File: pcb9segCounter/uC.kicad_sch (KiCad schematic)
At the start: 14 parts, among them J1 AVR-ISP-6, J2 SAO, U1 ATtiny84A-SS

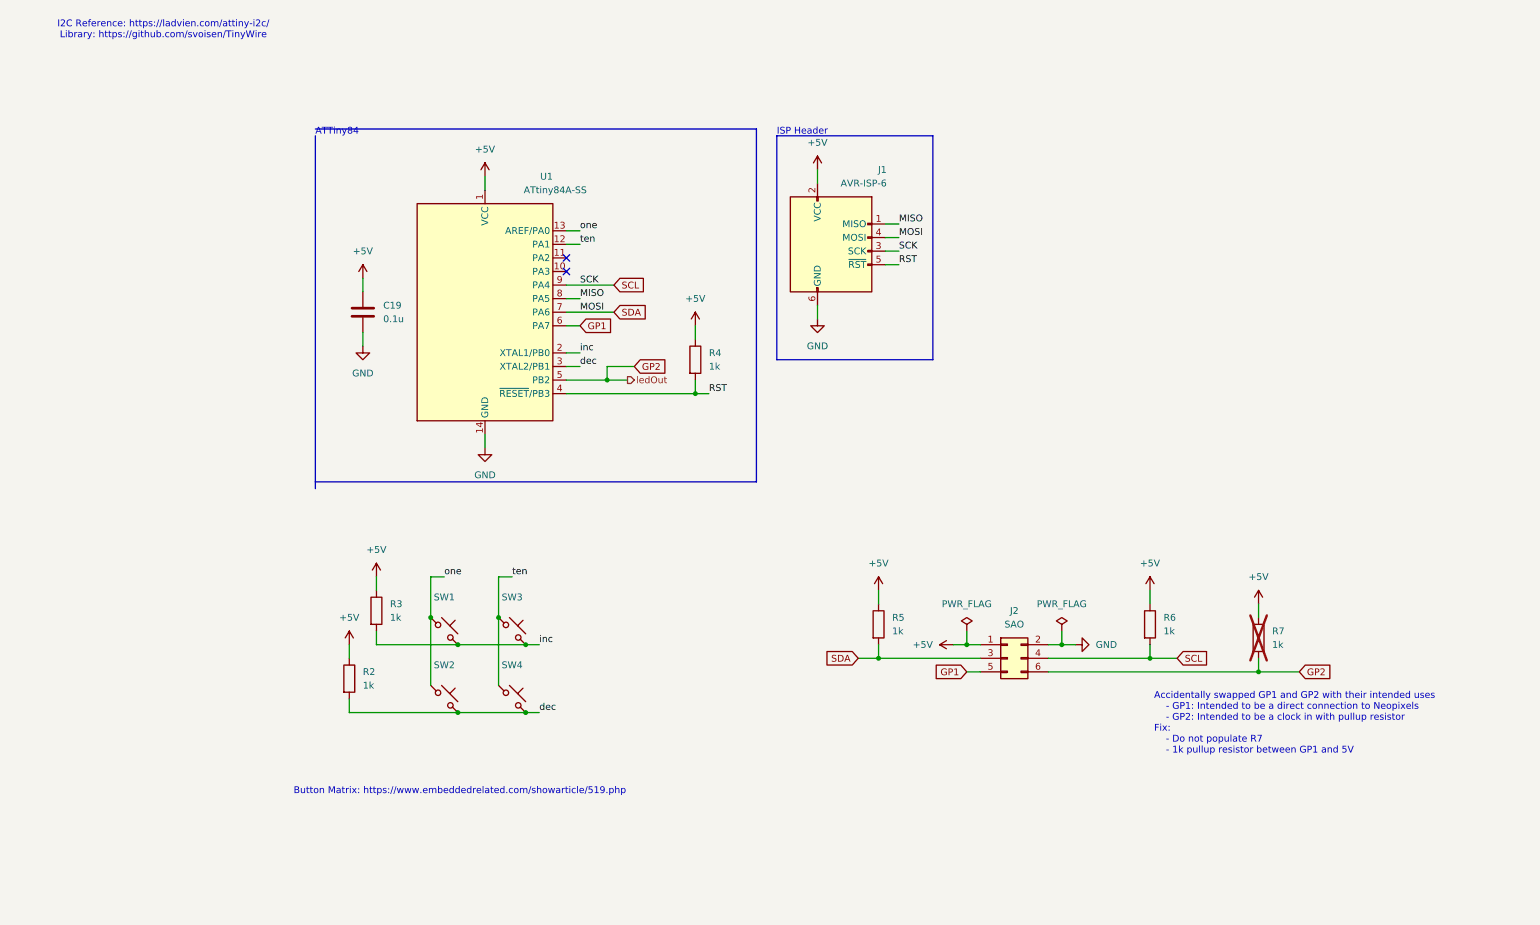
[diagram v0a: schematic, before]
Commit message: Doing lots of cleanup
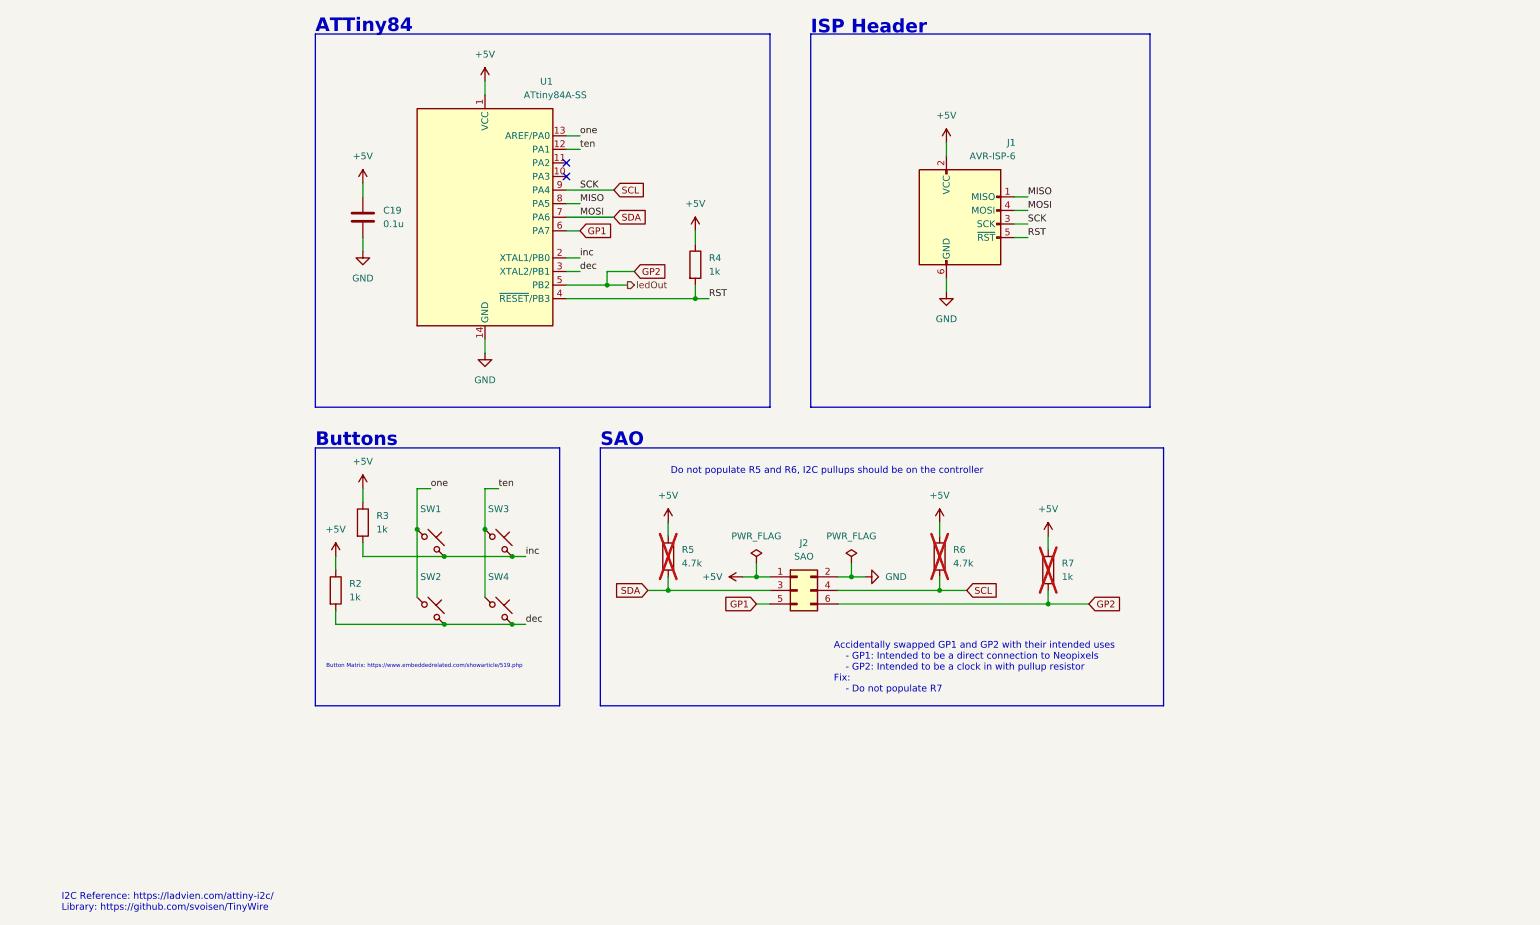
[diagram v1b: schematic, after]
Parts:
- R5, R6: value 1k -> 4.7k; now not fitted
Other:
- note added: "Accidentally swapped GP1 and GP2 with their intended uses - GP1: Intended to be a direct connection to Neopixels - GP2: Intended to be a clock in with pullup resistor Fix: - Do not populate R7"
- note added: "Buttons"
- note added: "Do not populate R5 and R6, I2C pullups should be on the controller"
- note added: "SAO"
- note removed: "Accidentally swapped GP1 and GP2 with their intended uses - GP1: Intended to be a direct connection to Neopixels - GP2: Intended to be a clock in with pullup resistor Fix: - Do not populate R7 - 1k pullup resistor between GP1 and 5V"
- company: (none) -> Ryan Martin
- title: (none) -> Nine Segment SAO
- moved on the sheet: C19, J1, J2, R2, R3, R4, R7, SW1, SW2, SW3, SW4, U1
